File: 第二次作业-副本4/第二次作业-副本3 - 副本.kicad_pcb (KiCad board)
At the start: 2 copper layers, 69.1 x 88.3 mm, 51 parts, among them J1 USB_C_Receptacle_USB2.0, J2 Conn_01x04, J3 Conn_01x02, J4 Conn_01x19, J5 Conn_01x20, J6 Conn_01x02, J7 Conn_01x03, Q1 Q_PMOS_DGS, SW1 SW_Push, SW2 SW_Push, SW3 SW_Push, SW4 SW_Push, U1 HX9193, U2 TJA1051T-3, U3 CH340E, U4 STM32F103C8Tx, U5 AD8400ARZ50, Y1 12M

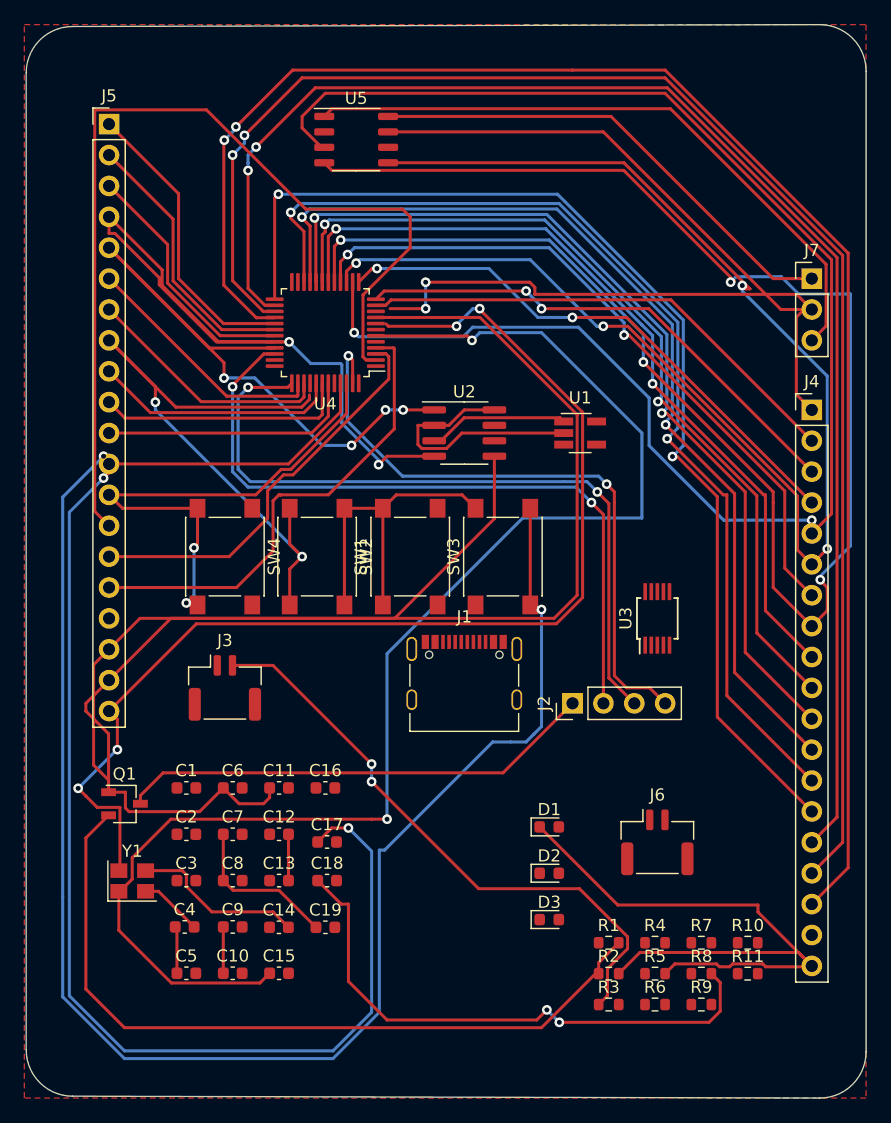
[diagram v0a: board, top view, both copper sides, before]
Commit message: youhua
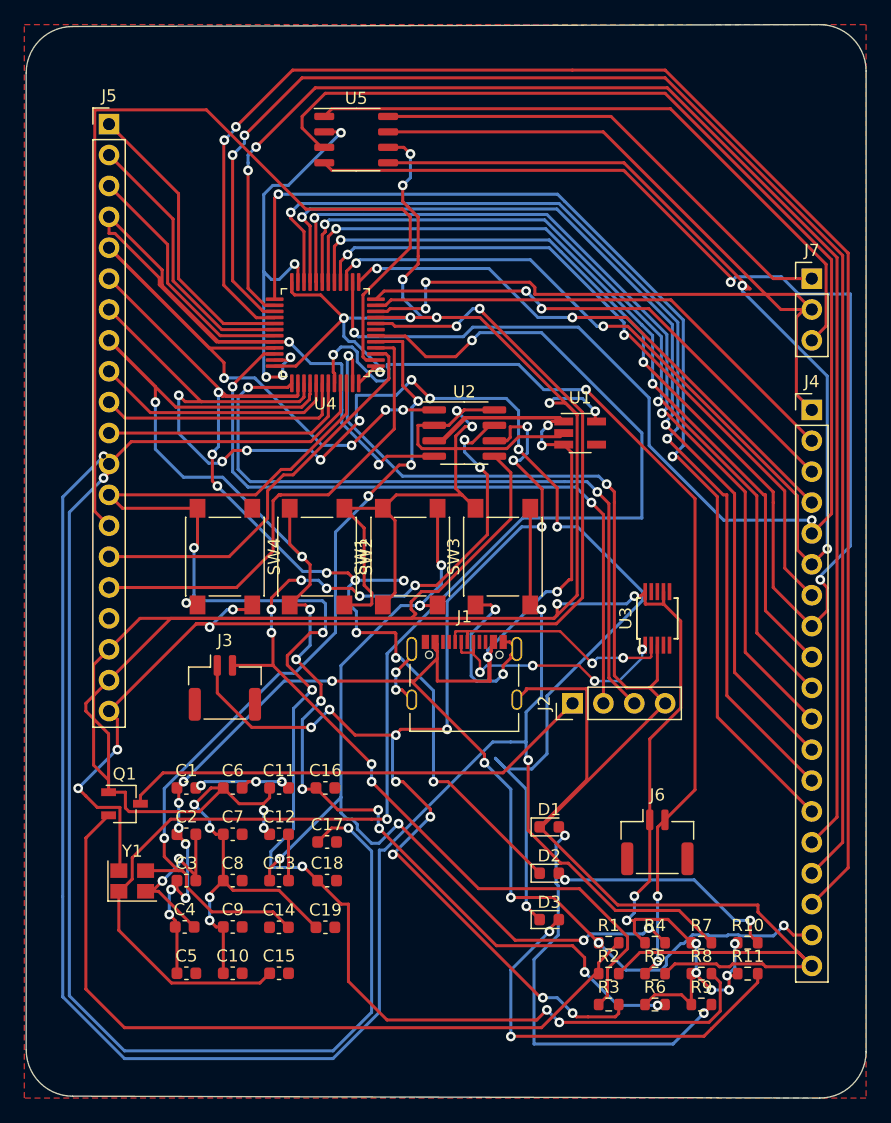
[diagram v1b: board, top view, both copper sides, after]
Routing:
- net +3V3: track 174.8 -> 320.9 mm, vias 0 -> 25
- net VBUS: track 14.9 -> 158.5 mm, vias 0 -> 16
- net GND: track 263.1 -> 394.7 mm, vias 6 -> 24
- net /STM32_MinimumSystem/PB3: track 20.5 -> 117.4 mm, vias 0 -> 10
- net Net-(J3-Pad1): track 0.00 -> 96.9 mm, vias 0 -> 12
- net /STM32_MinimumSystem/BOOTO: track 0.00 -> 80.8 mm, vias 0 -> 4
- net /STM32_MinimumSystem/NRST: track 0.00 -> 73.7 mm, vias 0 -> 7
- net /STM32_MinimumSystem/PA15: track 20.6 -> 87.6 mm, vias 0 -> 9
- net /STM32_MinimumSystem/PB4: track 52.5 -> 113.3 mm, vias 2 -> 10
- net /STM32_MinimumSystem/OSC_IN: track 14.2 -> 71.7 mm, vias 0 -> 4
- net /STM32_MinimumSystem/PB9: track 87.8 -> 129.9 mm, vias 4 -> 7
- net Net-(J3-Pad2): track 49.1 -> 87.5 mm, vias 2 -> 10
- net Net-(D1-Pad2): track 0.00 -> 35.2 mm, vias 0 -> 2
- net Net-(D3-Pad2): track 0.00 -> 34.1 mm, vias 0 -> 2
- net /STM32_MinimumSystem/PB8: track 241.1 -> 267.4 mm, vias 4 -> 5
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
